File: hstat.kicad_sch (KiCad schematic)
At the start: 78 parts, among them J1 BAT, J3 TMP2, J4 OUT-1, J5 OUT-2, J6 USB_C_Receptacle_USB2.0_16P, K1 EE2-3TNUH, Q1 AO3401A, Q2 BC817-40, Q3 BC817-40, Q4 BC817-40, Q5 BC817-40, SW1 SW_Push, SW2 SW_Push, SW3 SW_Push, SW4 SW_Push, SW5 SW_Push, U1 TP4057, U2 SY8089AAAC, U3 ESP32-WROVER-E, U4 CH340T, U5 BME280, U6 EL817, U7 EL817, Y1 12MHz

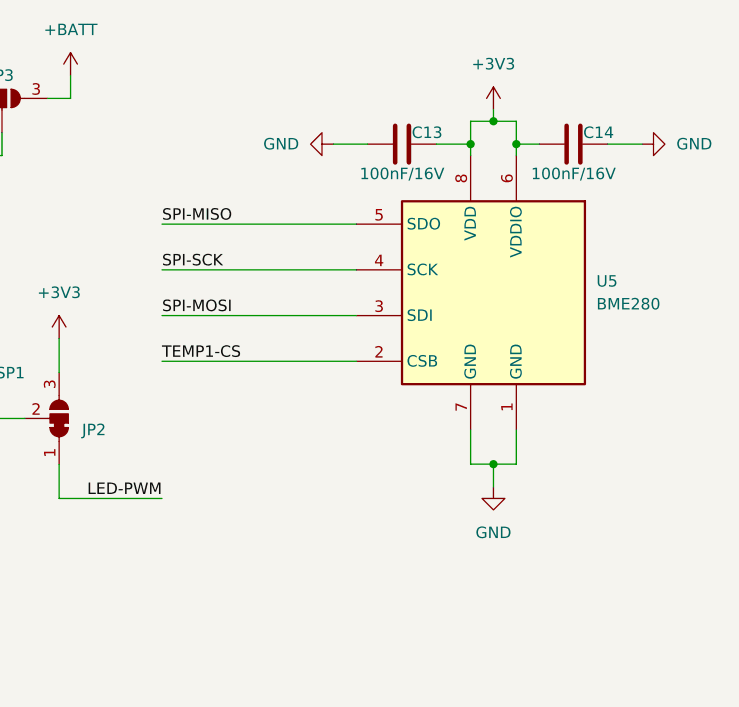
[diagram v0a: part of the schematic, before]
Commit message: new schematic
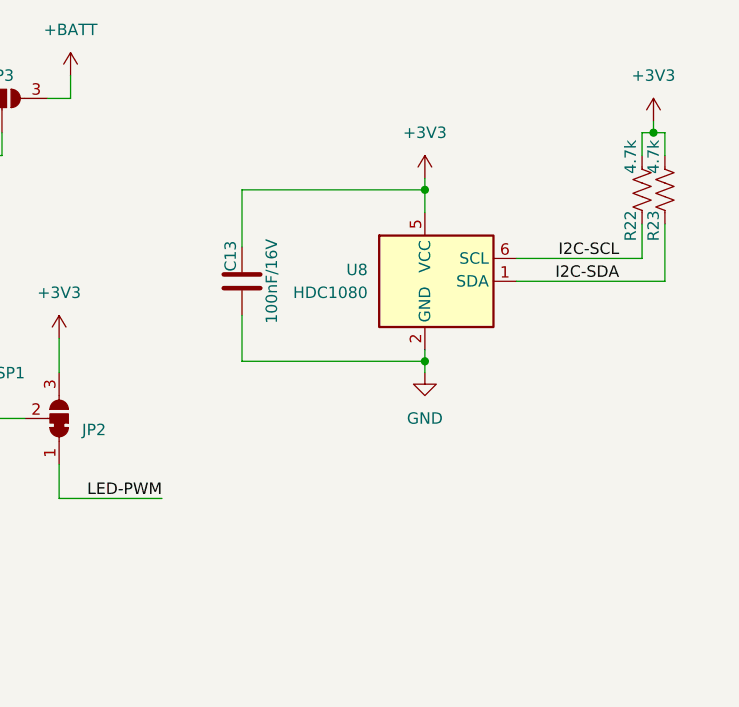
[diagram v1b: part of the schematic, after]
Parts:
- removed C14: 100nF/16V, Capacitor_SMD:C_0805_2012Metric, symbol Device:C
- removed U5: BME280, Package_LGA:Bosch_LGA-8_2.5x2.5mm_P0.65mm_ClockwisePinNumbering, symbol Sensor:BME280
- added R22, R23: 4.7k, Resistor_SMD:R_0805_2012Metric, symbol Device:R_US
- added U8: HDC1080, Package_SON:Texas_PWSON-N6, symbol Sensor_Humidity:HDC1080
- C1, C2: LCSC C15850 -> (none)
- C10, C9: LCSC C107045 -> (none)
- C11, C3, C4, C5: LCSC C45783 -> (none)
- C12, C13, C6, C7: LCSC C28233 -> (none)
- C15, C16: LCSC C116241 -> (none)
- C8: LCSC C15849 -> (none)
- D1: LCSC C191023 -> (none)
- D2, D3, D4: LCSC C8598 -> (none)
- D5: LCSC C37704 -> (none)
- D6, D7: LCSC C95872 -> (none)
- L1: LCSC C5832372 -> (none)
- LED1: LCSC C2297 -> (none)
- LED2: LCSC C84256 -> (none)
- LED3: LCSC C2296 -> (none)
- Q1: LCSC C15127 -> (none)
- Q2, Q3, Q4, Q5: LCSC C20069155 -> (none)
- R1, R10, R11, R19, R21: LCSC C17513 -> (none)
- R12, R14, R15, R16, R17, R6, R8, R9: LCSC C17414 -> (none)
- R13, R18, R20, R7: LCSC C17557 -> (none)
- R3, R4: LCSC C17556 -> (none)
- R5: LCSC C17477 -> (none)
- SW1, SW2, SW3, SW4, SW5: LCSC C318884 -> (none)
- U1: footprint Package_TO_SOT_SMD:TSOT-23-6 -> Package_TO_SOT_SMD:SOT-23-6; LCSC C12044 -> (none)
- U2: LCSC C78988 -> (none)
- U3: LCSC C2973667 -> (none)
- U4: LCSC C8689 -> (none)
- U6, U7: LCSC C106900 -> (none)
- Y1: LCSC C9002 -> (none)
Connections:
- net +3V3: now also R22.1, R23.1, U8.5 (VCC)
- net GND: now also U8.2 (GND)
- net I2C-SCL: now also R22.2, U8.6 (SCL)
- net I2C-SDA: now also R23.2, U8.1 (SDA)
